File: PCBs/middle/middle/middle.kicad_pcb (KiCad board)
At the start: 2 copper layers, 95.1 x 95.1 mm, 27 parts, among them J15 Screw_Terminal_01x02, J16 Screw_Terminal_01x02, J17 Screw_Terminal_01x02, J18 Screw_Terminal_01x02, J19 Screw_Terminal_01x02, J2 Screw_Terminal_01x03, J21 Screw_Terminal_01x02, J3 Screw_Terminal_01x03, J4 Screw_Terminal_01x03, J5 Screw_Terminal_01x03, SW1 SW_Push, SW2 SW_Push, SW3 SW_Push, U1 DEV-16771, U2 4754, U3 RFM69HCW

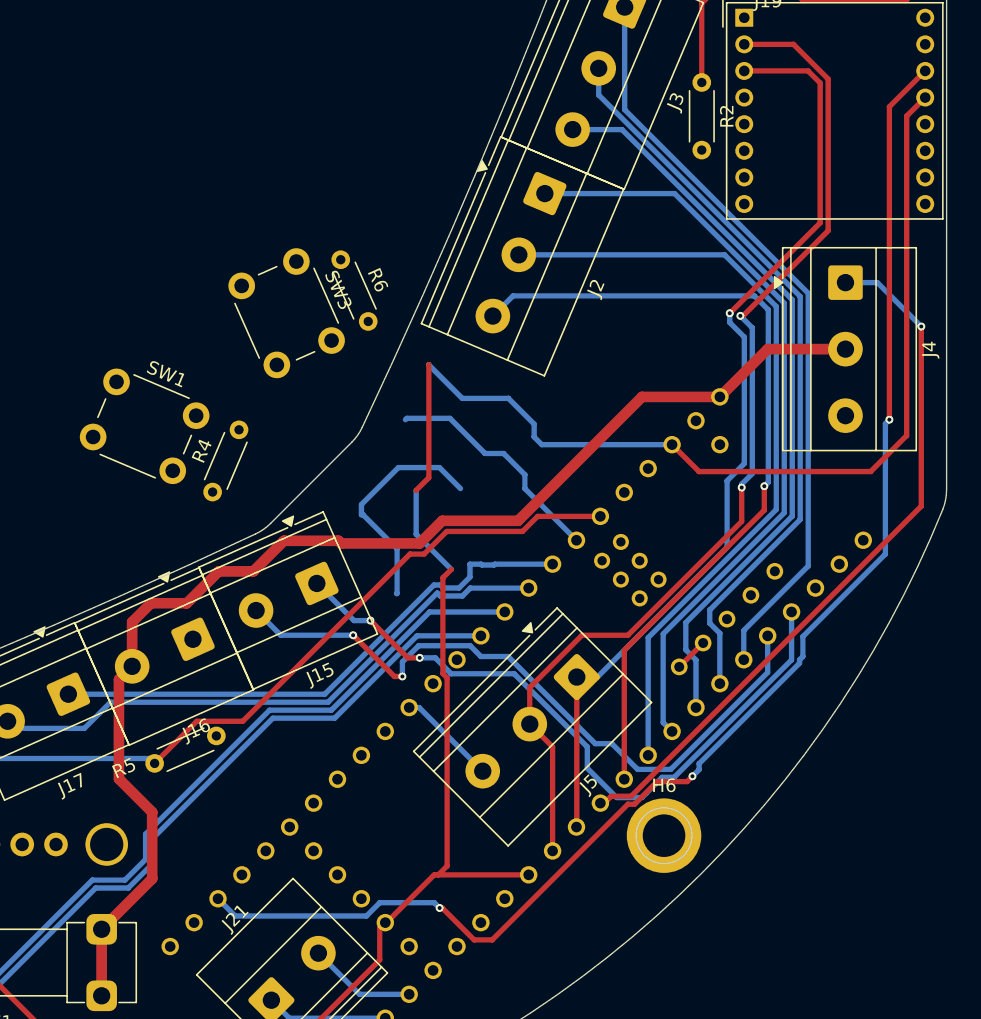
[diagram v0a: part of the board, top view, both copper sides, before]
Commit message: middle update
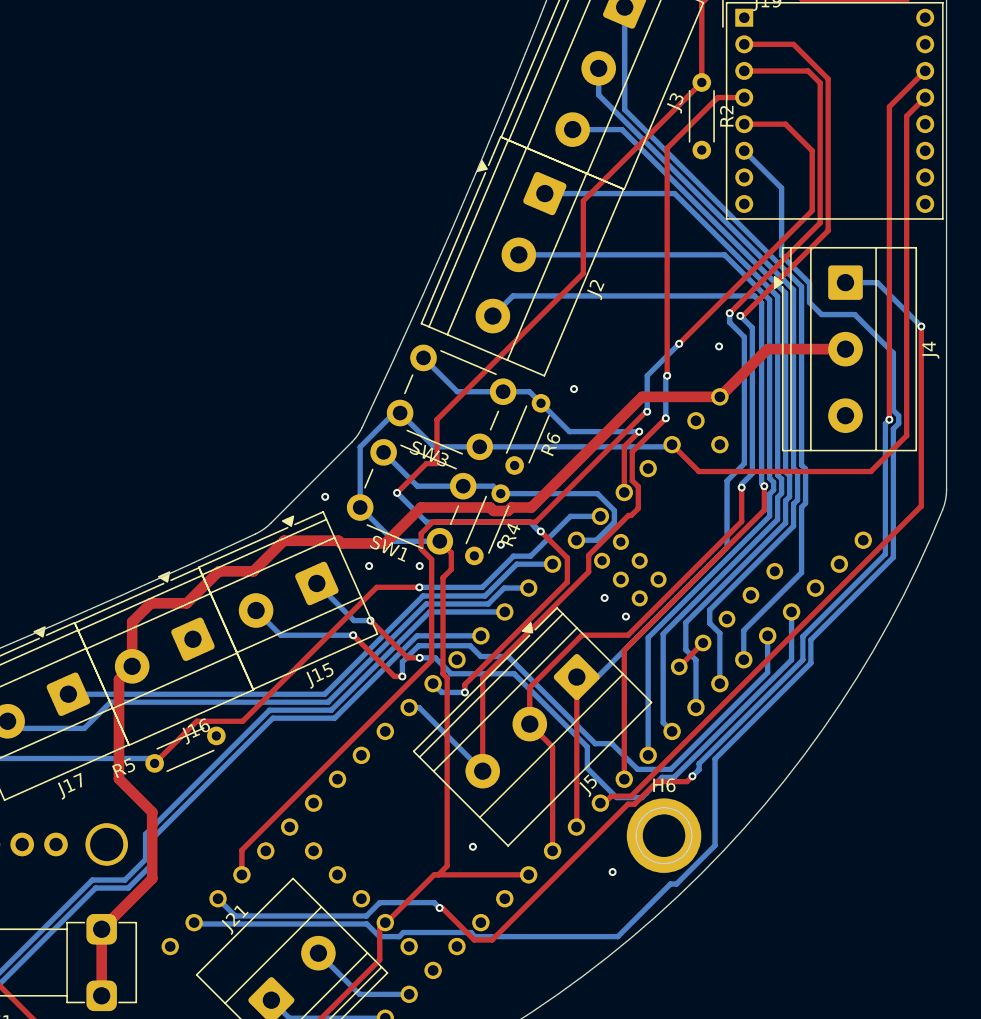
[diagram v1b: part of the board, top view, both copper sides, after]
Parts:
- moved SW1 27.1 mm to (159.7, 93.5), turned to 157 degrees
- moved R4 21.7 mm to (164.3, 90.0), turned to -113 degrees
- moved SW3 19.6 mm to (162.7, 86.4), turned to 157 degrees
- moved R6 18.5 mm to (167.3, 83.2), turned to -113 degrees
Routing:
- net /RFMreset: track 0.00 -> 106.9 mm
- net /NSS: track 0.00 -> 83.3 mm, vias 0 -> 2
- net /Vbat: track 25.2 -> 97.3 mm, vias 0 -> 3
- net /SCLK: track 7.51 -> 67.9 mm, vias 0 -> 2
- net Net-(U1-A8): track 17.2 -> 23.5 mm, vias 0 -> 1
- net Net-(U1-A6): track 17.3 -> 23.4 mm
- net +3.3V: track 196.2 -> 197.6 mm
- net /SCL1: track 41.2 -> 40.4 mm
- net Net-(U1-A7): track 63.4 -> 63.5 mm, vias 0 -> 1
- net GND: vias 0 -> 10
